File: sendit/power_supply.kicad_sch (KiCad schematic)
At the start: 42 parts, among them J58 JUMPER, J59 Conn_01x02, U11 AP63205WU, U7 TPS7A2033PDBVR, U8 TPS61040DBV

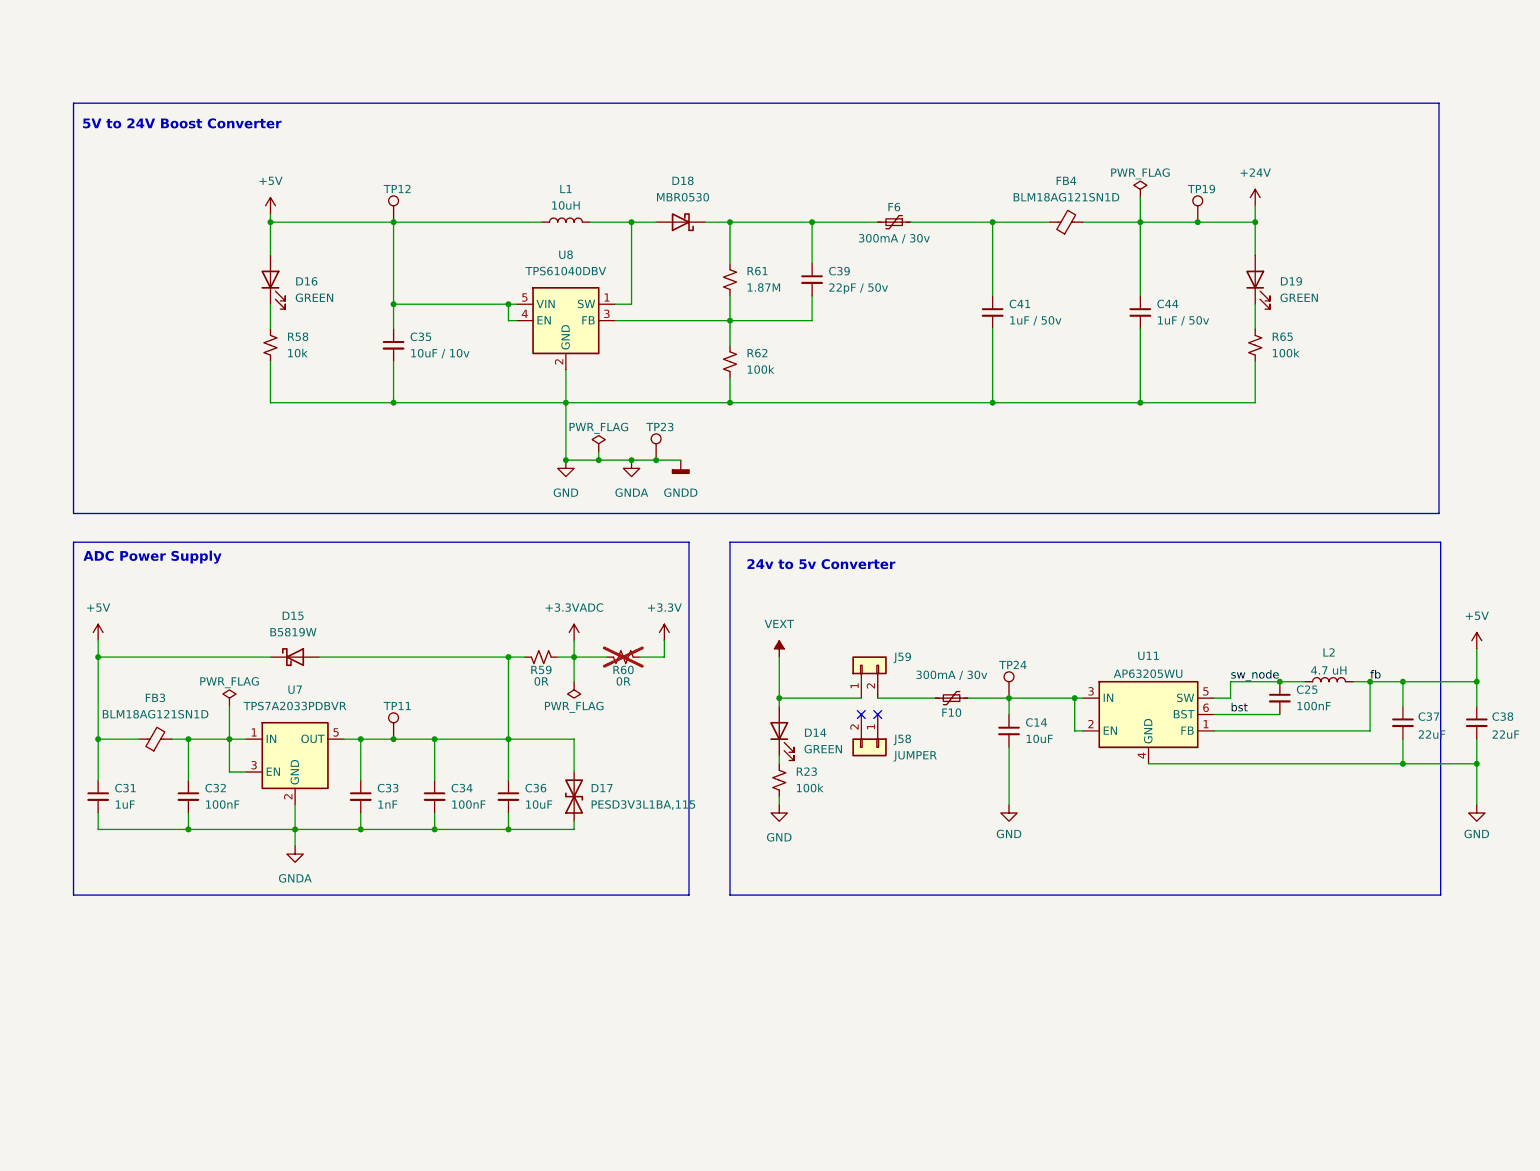
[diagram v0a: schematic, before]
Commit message: most of the work on the schematic is done.
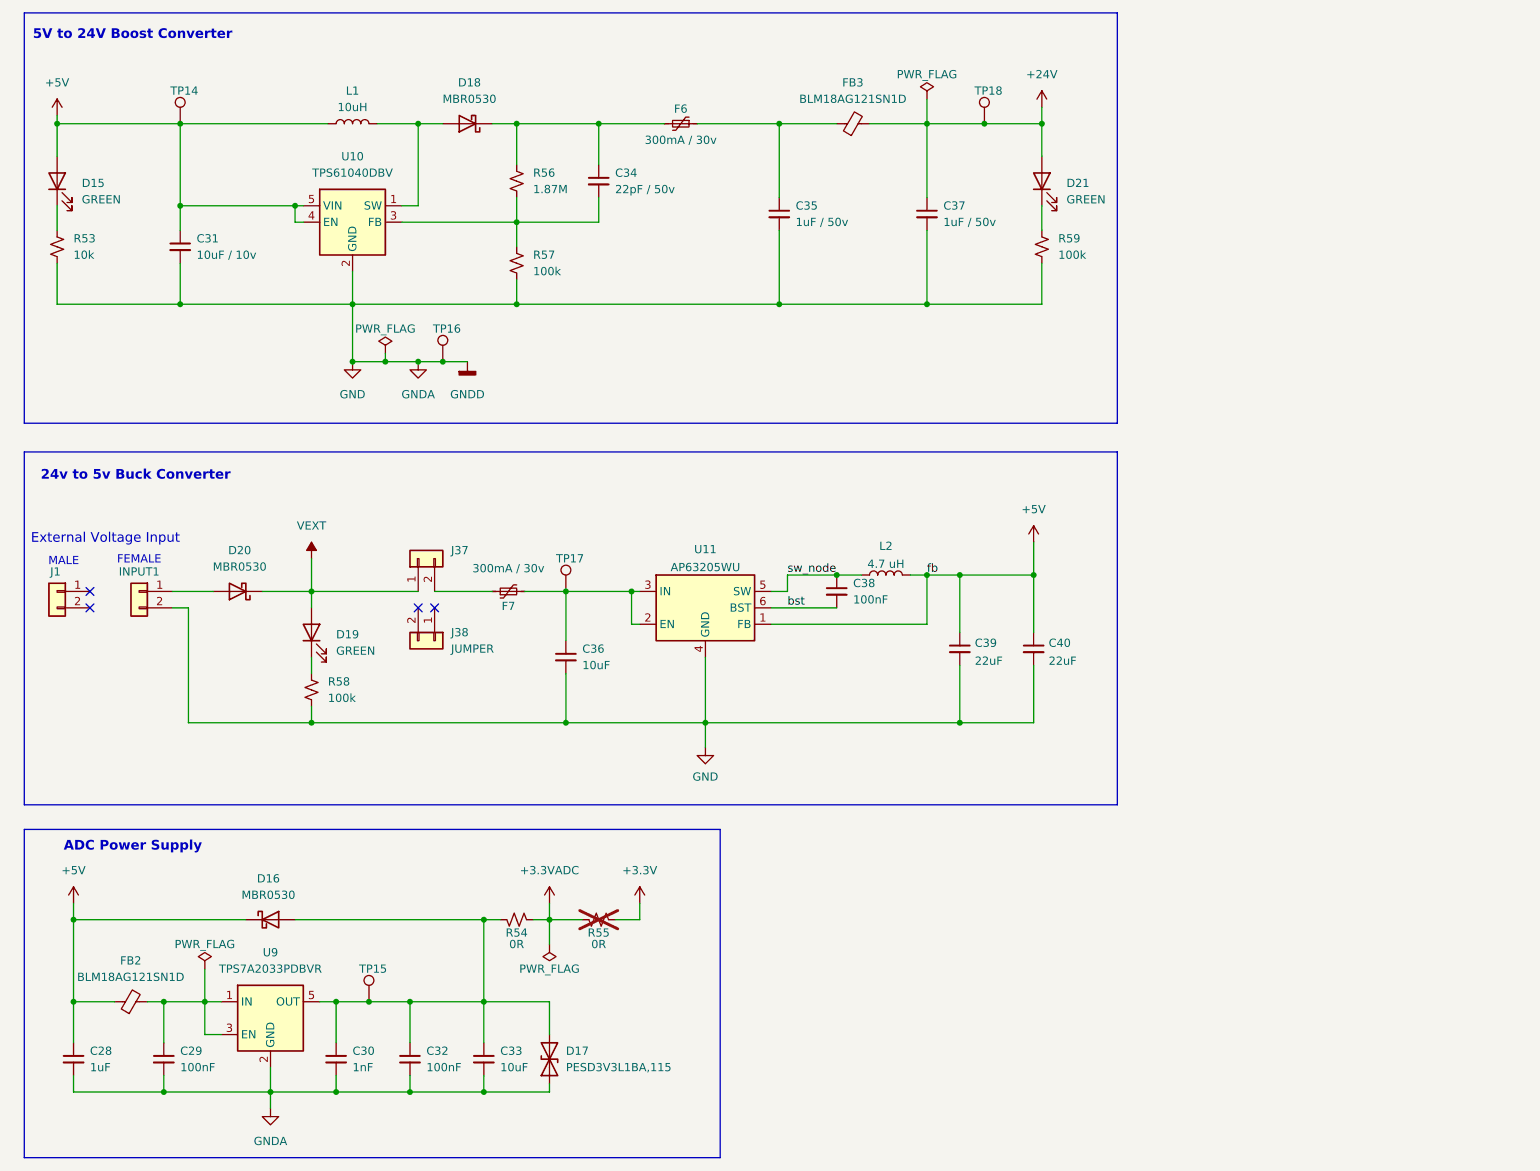
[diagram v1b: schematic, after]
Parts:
- removed D15: B5819W, Diode_SMD:D_SOD-123, symbol Device:D_Schottky
- added D16, D20: MBR0530, Diode_SMD:D_SOD-123, symbol Diode:MBR0530
- added INPUT1: Conn_01x02, yarrboard:PhoenixContact_MC_1,5_2-G-3.5_1x02_P3.50mm_Horizontal, symbol Connector_Generic:Conn_01x02
- added J1: Conn_01x02, symbol Connector_Generic:Conn_01x02
- L2: footprint Inductor_SMD:CKCS3010 -> Inductor_SMD:L_Neosid_SMS-ME3010
- U11: footprint Package_TO_SOT_SMD:TSOT-26 -> Package_TO_SOT_SMD:TSOT-23-6
- renumbered C31 to C28, C32 to C29, C33 to C30, C35 to C31, C34 to C32, C36 to C33, C39 to C34, C41 to C35, C14 to C36, C44 to C37, C25 to C38, C37 to C39, C38 to C40, D16 to D15, D14 to D19, D19 to D21, F10 to F7, FB3 to FB2, FB4 to FB3, J59 to J37, J58 to J38, R58 to R53, R59 to R54, R60 to R55, R61 to R56, R62 to R57, R23 to R58, R65 to R59, TP12 to TP14, TP11 to TP15, TP23 to TP16, TP24 to TP17, TP19 to TP18, U8 to U10, U7 to U9
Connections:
- net +5V: now also D16.1 (K)
- net GND: now also INPUT1.2 (Pin_2)
- net VEXT: now also D20.1 (K)
- net at C30.1, C32.1, C33.1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: now also D16.2 (A)
- new net: D20.2 (A), INPUT1.1 (Pin_1)
- no-connect marks 2 -> 4
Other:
- note added: "24v to 5v Buck Converter"
- note added: "External Voltage Input"
- note added: "FEMALE"
- note added: "MALE"
- note removed: "24v to 5v Converter"
- moved on the sheet: C28, C29, C30, C31, C32, C33, C34, C35, C36, C37, C38, C39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
